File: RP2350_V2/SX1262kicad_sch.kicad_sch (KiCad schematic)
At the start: 28 parts, among them J2 901-143-6RFX

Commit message: initial Transceiver layout
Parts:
- J2: LCSC (none) -> C429844
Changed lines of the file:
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@@
+			)
+		)
+		(property "LCSC" "C429844"
+			(at 276.86 78.74 0)
+			(effects
+				(font
+					(size 1.27 1.27)
+				)
+				(hide yes)
 			)
 		)

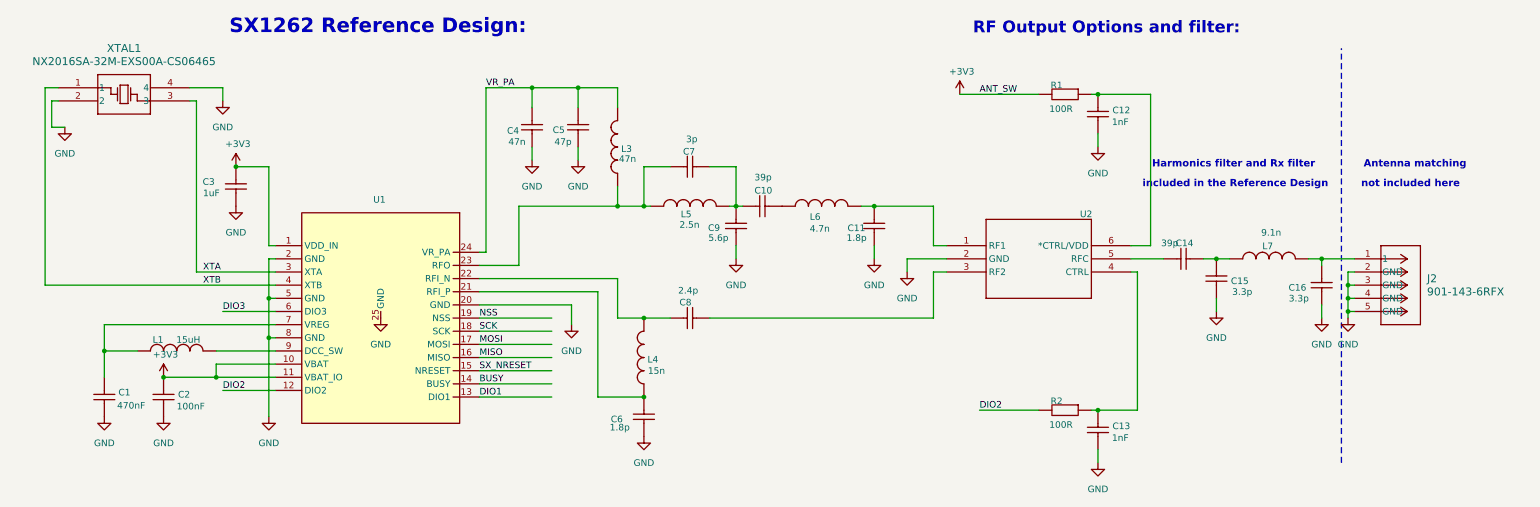
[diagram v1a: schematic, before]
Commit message: progress :D
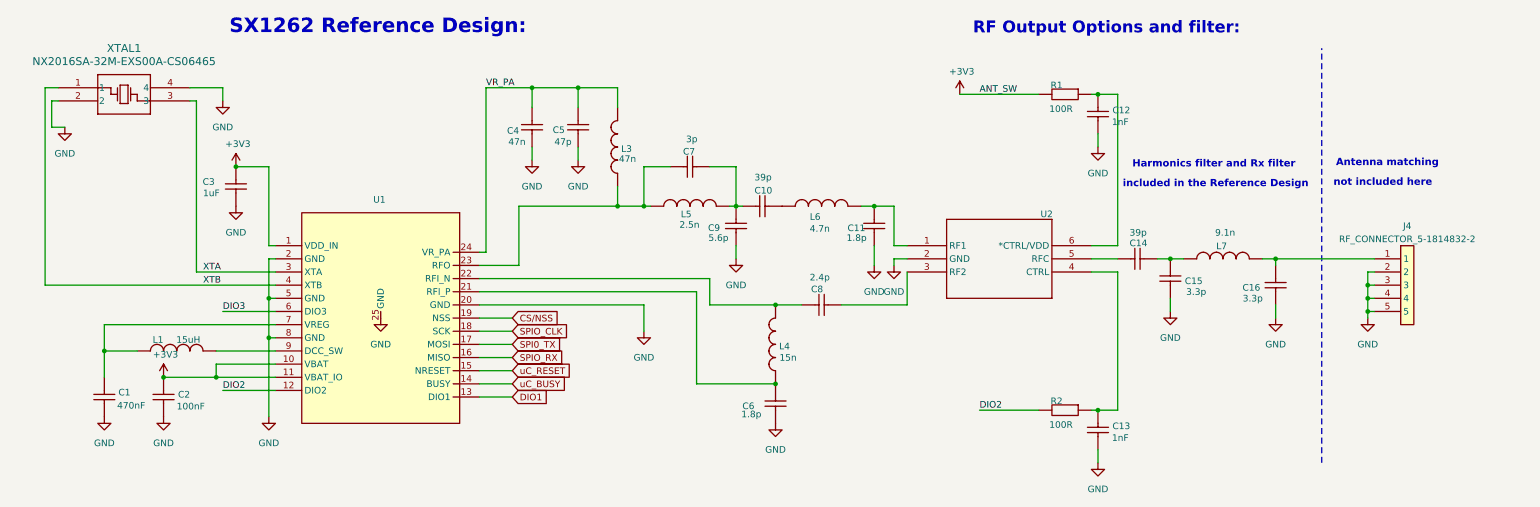
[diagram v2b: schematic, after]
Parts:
- removed J2: 901-143-6RFX, My_Footprints:RF_ANT_OUTPUT_901-143-6RFX, symbol My_Library:901-143-6RFX
- added J4: RF_CONNECTOR_5-1814832-2, My_Footprints:RF_CONNECTOR_518148322, symbol My_Library:RF_CONNECTOR_5-1814832-2
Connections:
- net GND: now also J4.2, J4.3, J4.4, J4.5
- net at C16.2, L7.2: now also J4.1
- net BUSY renamed uC_BUSY
- net MISO renamed SPIO_RX
- net MOSI renamed SPI0_TX
- net NSS renamed CS/NSS
- net SCK renamed SPIO_CLK
- net SX_NRESET renamed uC_RESET
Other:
- moved on the sheet: C14, C15, C16, C6, C8, L4, L7, U2
